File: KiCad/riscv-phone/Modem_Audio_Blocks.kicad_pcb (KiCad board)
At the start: 2 copper layers, 45.9 x 62.2 mm, 46 parts, among them J1 Conn_01x08, J10 SIM_Card, J2 Conn_01x02, J3 Conn_01x05, J4 Conn_02x03_Odd_Even, J5 Conn_01x02, J6 Conn_01x02, J7 Conn_01x02, J8 Conn_01x02, J9 SJ-3524-SMT, Q1 MMBT3904, U1 NAU8810, U2 TXS0108EPW, U3 uBlox_TOBY-R200, U4 TXS0108EPW

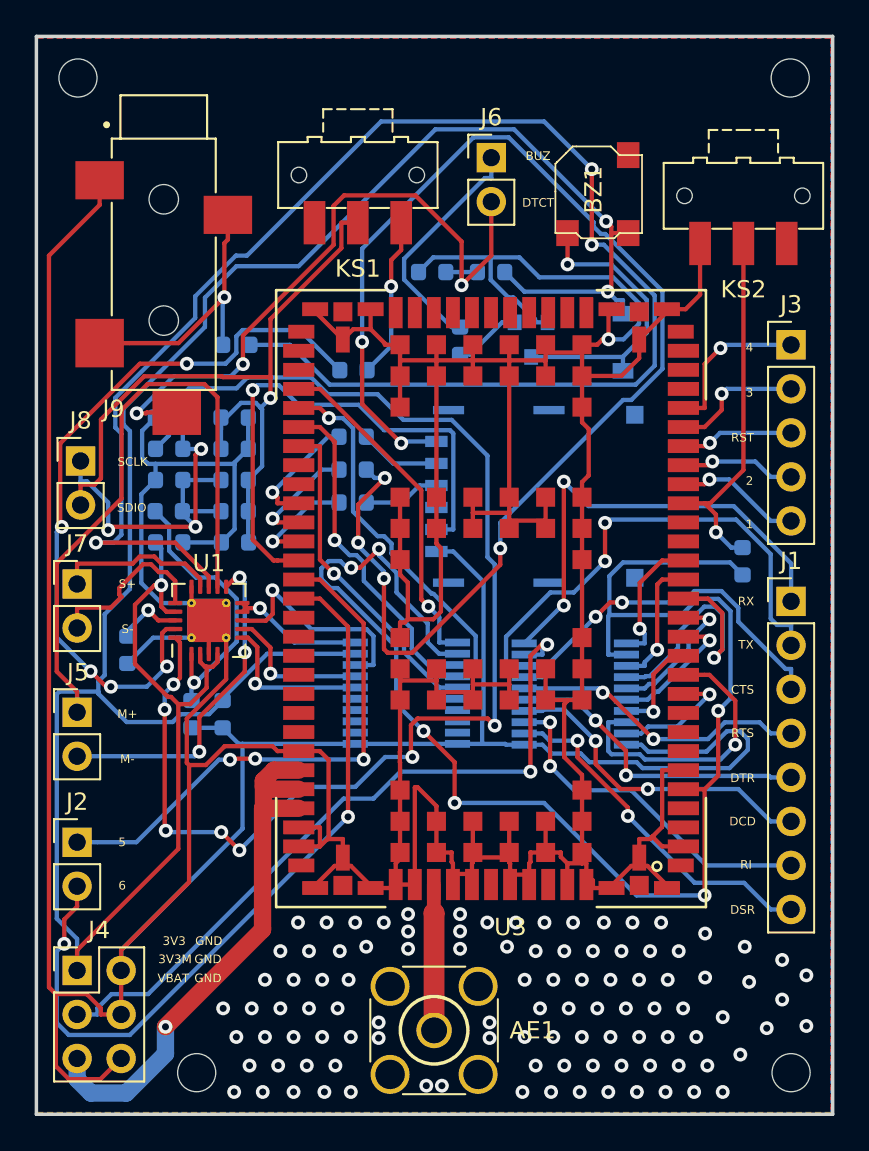
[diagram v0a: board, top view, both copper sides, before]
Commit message: Final PCB with added changes
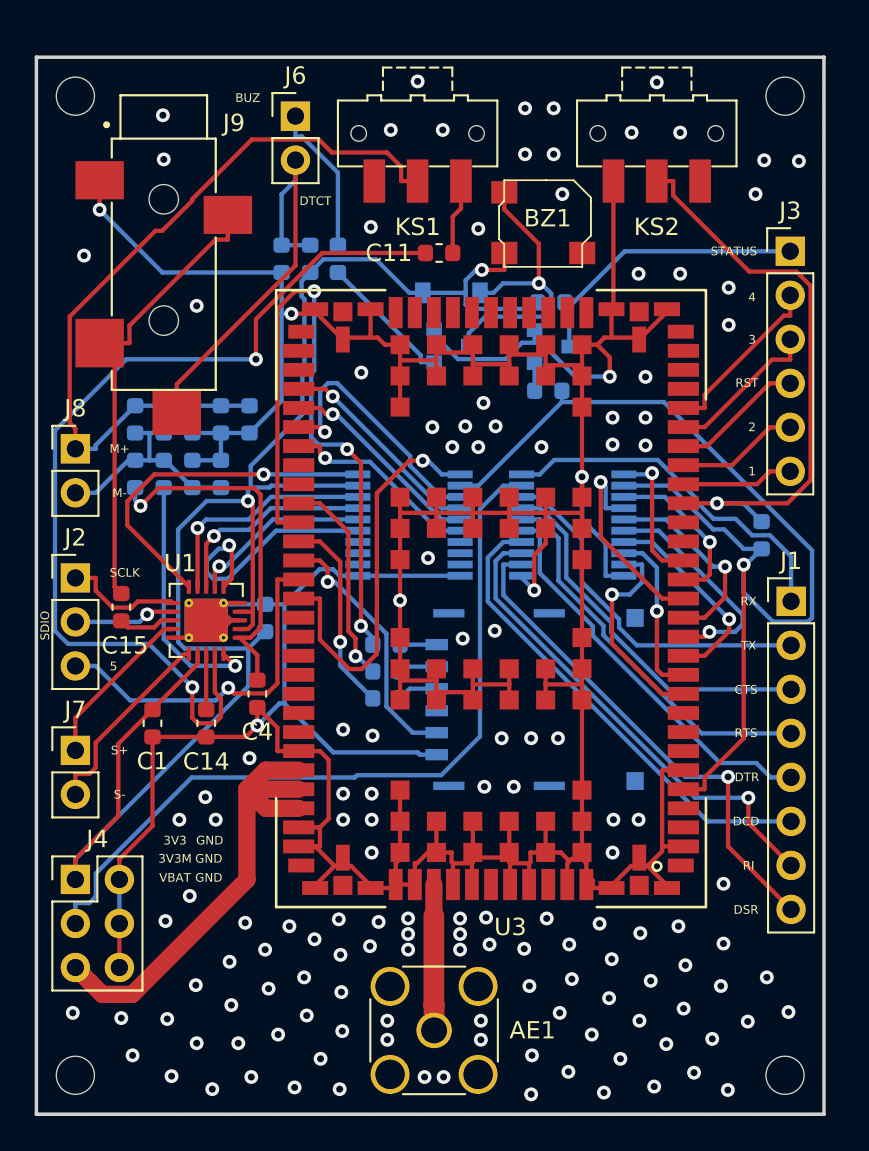
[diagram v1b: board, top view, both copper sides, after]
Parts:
- removed ? (x4): MountingHole_2.2mm_M2_ISO7380, MountingHole:MountingHole_2.2mm_M2_ISO7380
- removed J5: Conn_01x02, Connector_PinHeader_2.54mm:PinHeader_1x02_P2.54mm_Vertical
- added Q2: MMBT3904, Package_TO_SOT_SMD:SOT-23, B.Cu at (133.4, 81.7)
- added R11: 1k, Resistor_SMD:R_0603_1608Metric, B.Cu at (133.4, 79.2)
- added R9: 1k, Resistor_SMD:R_0603_1608Metric, B.Cu at (133.2, 84.2)
- added m1: MountingHole_2.2mm_M2_ISO7380, MountingHole:MountingHole_2.2mm_M2_ISO7380, F.Cu at (146.8, 67.2)
- added m2: MountingHole_2.2mm_M2_ISO7380, MountingHole:MountingHole_2.2mm_M2_ISO7380, F.Cu at (105.9, 67.2)
- added m3: MountingHole_2.2mm_M2_ISO7380, MountingHole:MountingHole_2.2mm_M2_ISO7380, F.Cu at (105.9, 123.8)
- added m4: MountingHole_2.2mm_M2_ISO7380, MountingHole:MountingHole_2.2mm_M2_ISO7380, F.Cu at (146.8, 123.8)
- C1, C11, C14, C15, C4: moved to F.Cu
- J2: value Conn_01x02 -> Conn_01x03; footprint Connector_PinHeader_2.54mm:PinHeader_1x02_P2.54mm_Vertical -> Connector_PinHeader_2.54mm:PinHeader_1x03_P2.54mm_Vertical
- J3: value Conn_01x05 -> Conn_01x06; footprint Connector_PinHeader_2.54mm:PinHeader_1x05_P2.54mm_Vertical -> Connector_PinHeader_2.54mm:PinHeader_1x06_P2.54mm_Vertical
- moved C15 16.5 mm to (108.5, 96.7), turned to 270 degrees
- moved J2 15.3 mm to (105.9, 95.0)
- moved R6 13.7 mm to (123.8, 100.5)
- moved J10 11.7 mm to (129.1, 102.2)
- moved J6 11.6 mm to (118.6, 68.4)
- moved R8 11.5 mm to (123.8, 102.0)
- moved R4 10.5 mm to (119.5, 76.6), turned to 90 degrees
- moved D1 10.3 mm to (127.6, 78.6), turned to 0 degrees
- moved R7 10.3 mm to (123.8, 98.9)
- moved U2 9.75 mm to (134.6, 92.0)
- moved U4 9.70 mm to (125.2, 92.0)
- moved J7 9.60 mm to (105.9, 105.0)
- moved C16 8.72 mm to (117.8, 76.6), turned to 270 degrees
- moved R1 8.49 mm to (121.0, 76.6)
- moved C11 8.37 mm to (126.9, 76.3)
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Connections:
- J2 pad 1: /ModemINDIV/GPIO5 -> /AudioINDIV/SCLK
- J2 pad 2: /ModemINDIV/GPIO6 -> /AudioINDIV/SDIO
- J3 pad 1: /ModemINDIV/GPIO4 -> /ModemINDIV/STATUS
- J3 pad 2: /ModemINDIV/GPIO3 -> /ModemINDIV/GPIO4
- J3 pad 3: /ModemINDIV/RESET_N_1V8 -> /ModemINDIV/GPIO3
- J3 pad 4: /ModemINDIV/GPIO2 -> /ModemINDIV/RESET_N_1V8
- J3 pad 5: /ModemINDIV/GPIO1 -> /ModemINDIV/GPIO2
- J8 pad 1: /AudioINDIV/oMIC+ -> /AudioINDIV/oMIC-
- J8 pad 2: /AudioINDIV/oMIC- -> /AudioINDIV/oMIC+
- U1 pad 10: /AudioINDIV/BCLK -> /AudioINDIV/MCLK
- U3 pad 60: /ModemINDIV/GPIO5 -> /GPIO5
- U4 pad 1: Net-(U3-Pad50) -> /ModemINDIV/GPIO6
- U4 pad 15: Net-(U4-Pad15) -> /AudioINDIV/ADCOUT
- U4 pad 16: /AudioINDIV/ADCOUT -> /AudioINDIV/DACIN
- U4 pad 17: /AudioINDIV/DACIN -> /AudioINDIV/FS
- U4 pad 18: /AudioINDIV/FS -> /AudioINDIV/BCLK
- U4 pad 20: /AudioINDIV/BCLK -> /AudioINDIV/MCLK
- U4 pad 3: Net-(U3-Pad51) -> Net-(U3-Pad52)
- U4 pad 4: Net-(U3-Pad52) -> Net-(U3-Pad50)
- U4 pad 5: Net-(U3-Pad53) -> Net-(U3-Pad51)
- U4 pad 6: Net-(U4-Pad6) -> Net-(U3-Pad53)
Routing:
- net GND: track 444.8 -> 315.4 mm, vias 103 -> 143
- net Net-(C15-Pad2): track 91.6 -> 3.29 mm, vias 3 -> 0
- net Net-(J10-Pad7): track 79.3 -> 2.11 mm, vias 6 -> 0
- net /AudioINDIV/MIC+: track 75.0 -> 14.5 mm, vias 7 -> 1
- net +3V3: track 141.5 -> 99.4 mm, vias 3 -> 2
- net Net-(R7-Pad1): track 6.59 -> 38.8 mm, vias 1 -> 3
- net /ModemINDIV/GPIO5: track 31.2 -> 0.00 mm, vias 3 -> 0
- net /AudioINDIV/SDIO: track 36.9 -> 5.86 mm, vias 0 -> 1
- net /ModemINDIV/VDD_1V8: track 86.1 -> 62.7 mm, vias 6 -> 1
- net /ModemINDIV/GPIO6: track 45.2 -> 23.1 mm, vias 2 -> 1
- net /GPIO5: track 0.00 -> 20.4 mm, vias 0 -> 1
- net /AudioINDIV/MCLK: track 0.00 -> 20.4 mm, vias 0 -> 1
- net /ModemINDIV/STATUS: track 0.00 -> 16.7 mm
- net Net-(J10-Pad1): track 31.1 -> 15.0 mm
- net /AudioINDIV/HEADPHONE_DETECT: track 40.3 -> 24.3 mm, vias 3 -> 0
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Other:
- board size 45.9 x 62.2 mm -> 45.4 x 61 mm
- board text added: "STATUS"
- board text removed: "6"
